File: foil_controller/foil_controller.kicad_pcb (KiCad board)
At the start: 2 copper layers, 90 x 110 mm, 18 parts, among them J1 programming_header, J2 pwr_in, J3 ultra sensor 1, J4 ultra sensor 1, SW1 SW_Push, SW2 SW_Push, SW3 SW_Push, SW4 SW_Push, U1 RS485_module, U2 L7805

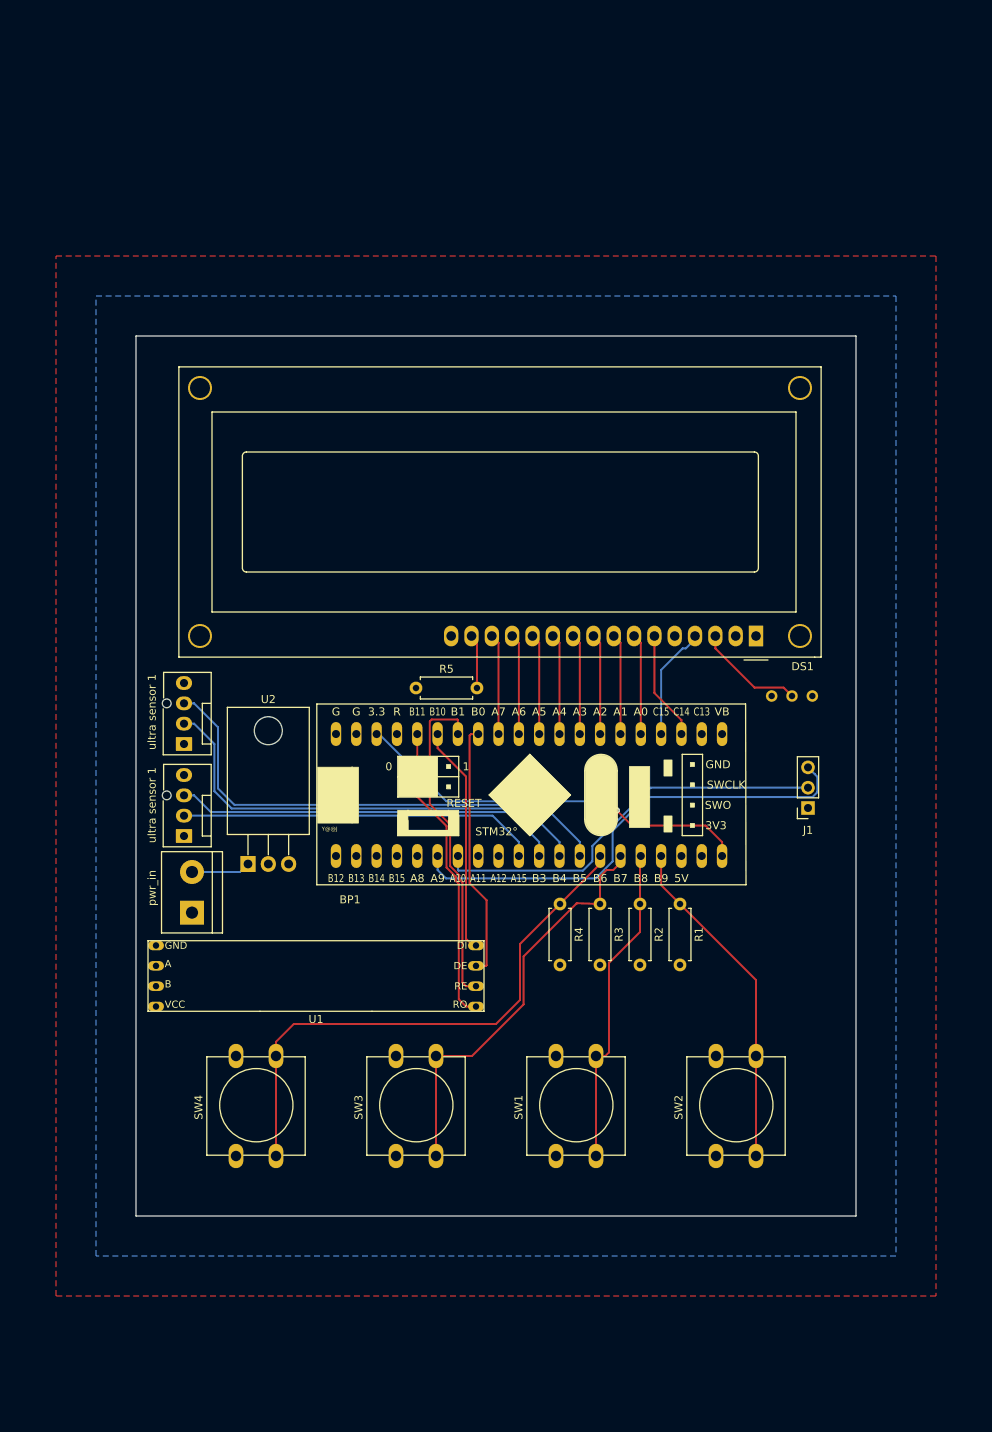
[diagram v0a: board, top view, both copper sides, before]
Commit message: controller v2 voor testvaart 1 mei
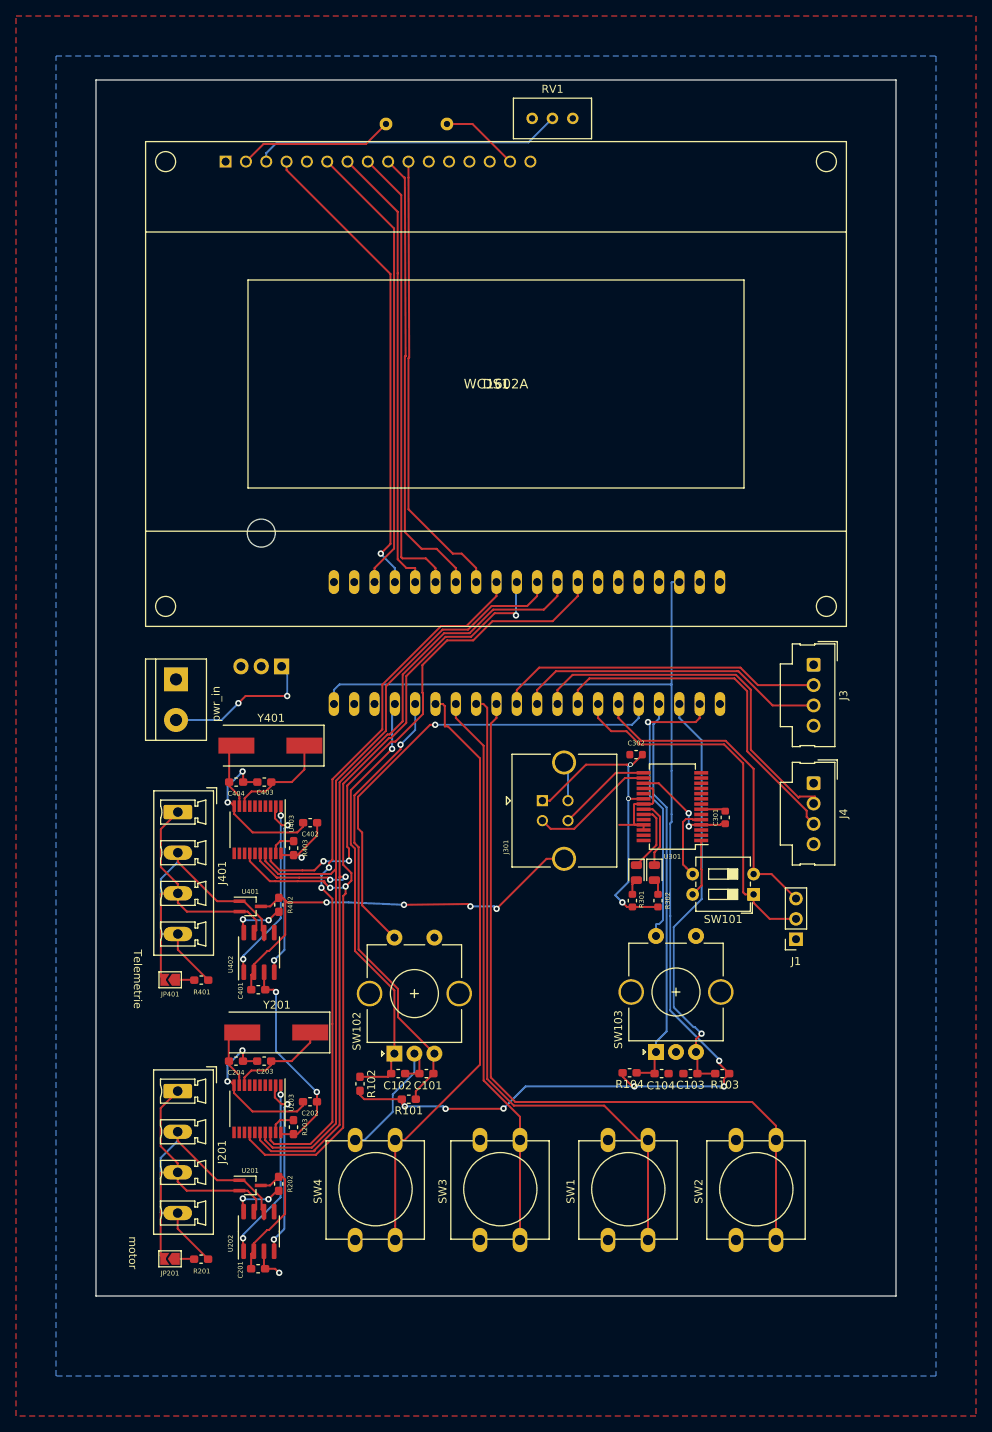
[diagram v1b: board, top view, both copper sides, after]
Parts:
- removed R1, R2, R3, R4: 10K, Resistor_THT:R_Axial_DIN0207_L6.3mm_D2.5mm_P7.62mm_Horizontal
- removed U1: RS485_module, stroom_shield:RS485_module
- added C101: 47nf, Capacitor_SMD:C_0603_1608Metric_Pad1.05x0.95mm_HandSolder, F.Cu at (36.3, 92.2)
- added C102: 47nf, Capacitor_SMD:C_0603_1608Metric_Pad1.05x0.95mm_HandSolder, F.Cu at (32.8, 92.2)
- added C103: 47nf, Capacitor_SMD:C_0603_1608Metric_Pad1.05x0.95mm_HandSolder, F.Cu at (69.3, 92.2)
- added C104: 47nf, Capacitor_SMD:C_0603_1608Metric_Pad1.05x0.95mm_HandSolder, F.Cu at (65.7, 92.2)
- added C201: 100nf, Capacitor_SMD:C_0603_1608Metric_Pad1.05x0.95mm_HandSolder, F.Cu at (15.3, 116.6)
- added C202: 100nf, Capacitor_SMD:C_0603_1608Metric_Pad1.05x0.95mm_HandSolder, F.Cu at (21.8, 95.7)
- added C203: 2pf, Capacitor_SMD:C_0603_1608Metric_Pad1.05x0.95mm_HandSolder, F.Cu at (16.0, 90.6)
- added C204: 2pf, Capacitor_SMD:C_0603_1608Metric_Pad1.05x0.95mm_HandSolder, F.Cu at (12.5, 90.6)
- added C301: 100nf, Capacitor_SMD:C_0603_1608Metric, F.Cu at (73.7, 60.2)
- added C302: 1uf, Capacitor_SMD:C_0603_1608Metric, F.Cu at (62.5, 52.3)
- added C401: 100nf, Capacitor_SMD:C_0603_1608Metric_Pad1.05x0.95mm_HandSolder, F.Cu at (15.3, 81.7)
- added C402: 100nf, Capacitor_SMD:C_0603_1608Metric_Pad1.05x0.95mm_HandSolder, F.Cu at (21.8, 60.8)
- added C403: 2pf, Capacitor_SMD:C_0603_1608Metric_Pad1.05x0.95mm_HandSolder, F.Cu at (16.0, 55.8)
- added C404: 2pf, Capacitor_SMD:C_0603_1608Metric_Pad1.05x0.95mm_HandSolder, F.Cu at (12.5, 55.8)
- added D301: TXLED, LED_SMD:LED_0805_2012Metric, F.Cu at (62.5, 67.1)
- added D302: RXLED, LED_SMD:LED_0805_2012Metric, F.Cu at (64.8, 67.1)
- added J201: can, Connector_Phoenix_MC_HighVoltage:PhoenixContact_MCV_1,5_4-G-5.08_1x04_P5.08mm_Vertical, F.Cu at (5.21, 94.4)
- added J301: USB_B, Connector_USB:USB_B_TE_5787834_Vertical, F.Cu at (50.8, 58.1)
- added J401: can, Connector_Phoenix_MC_HighVoltage:PhoenixContact_MCV_1,5_4-G-5.08_1x04_P5.08mm_Vertical, F.Cu at (5.23, 59.5)
- added JP201: termination, Jumper:SolderJumper-2_P1.3mm_Open_TrianglePad1.0x1.5mm, F.Cu at (4.25, 115.4)
- added JP401: termination, Jumper:SolderJumper-2_P1.3mm_Open_TrianglePad1.0x1.5mm, F.Cu at (4.27, 80.5)
- added R101: 10K, Resistor_SMD:R_0603_1608Metric_Pad1.05x0.95mm_HandSolder, F.Cu at (34.1, 95.4)
- added R102: 10K, Resistor_SMD:R_0603_1608Metric_Pad1.05x0.95mm_HandSolder, F.Cu at (28.0, 93.5)
- added R103: 10K, Resistor_SMD:R_0603_1608Metric_Pad1.05x0.95mm_HandSolder, F.Cu at (73.3, 92.2)
- added R104: 10K, Resistor_SMD:R_0603_1608Metric_Pad1.05x0.95mm_HandSolder, F.Cu at (61.7, 92.1)
- added R201: 120R, Resistor_SMD:R_0603_1608Metric_Pad1.05x0.95mm_HandSolder, F.Cu at (8.14, 115.4)
- added R202: 47K, Resistor_SMD:R_0603_1608Metric_Pad1.05x0.95mm_HandSolder, F.Cu at (17.8, 106.0)
- added R203: 10K, Resistor_SMD:R_0603_1608Metric_Pad1.05x0.95mm_HandSolder, F.Cu at (19.7, 98.9)
- added R301: 330R, Resistor_SMD:R_0603_1608Metric, F.Cu at (62.0, 70.6)
- added R302: 330R, Resistor_SMD:R_0603_1608Metric, F.Cu at (65.2, 70.6)
- added R401: 120R, Resistor_SMD:R_0603_1608Metric_Pad1.05x0.95mm_HandSolder, F.Cu at (8.16, 80.5)
- added R402: 47K, Resistor_SMD:R_0603_1608Metric_Pad1.05x0.95mm_HandSolder, F.Cu at (17.9, 71.1)
- added R403: 10K, Resistor_SMD:R_0603_1608Metric_Pad1.05x0.95mm_HandSolder, F.Cu at (19.7, 64.0)
- added SW101: SW_DIP_x02, Button_Switch_THT:SW_DIP_SPSTx02_Slide_6.7x6.64mm_W7.62mm_P2.54mm_LowProfile, F.Cu at (77.2, 69.8)
- added SW102: Encoder_1, Rotary_Encoder:RotaryEncoder_Alps_EC11E-Switch_Vertical_H20mm_CircularMountingHoles, F.Cu at (32.3, 89.7)
- added SW103: Encoder_2, Rotary_Encoder:RotaryEncoder_Alps_EC11E-Switch_Vertical_H20mm_CircularMountingHoles, F.Cu at (65.0, 89.5)
- added U201: PESD5V0L2UU_esd_diode, Package_TO_SOT_SMD:SOT-323_SC-70_Handsoldering, F.Cu at (14.3, 106.2)
- added U202: MCP2551-I-SN, Package_SO:SOIC-8_3.9x4.9mm_P1.27mm, F.Cu at (15.4, 111.9)
- added U203: MCP2515-xST, Package_SO:TSSOP-20_4.4x6.5mm_P0.65mm, F.Cu at (15.2, 96.6)
- added U301: FT232RL, Package_SO:SSOP-28_5.3x10.2mm_P0.65mm, F.Cu at (67.0, 58.8)
- added U401: PESD5V0L2UU_esd_diode, Package_TO_SOT_SMD:SOT-323_SC-70_Handsoldering, F.Cu at (14.3, 71.3)
- added U402: MCP2551-I-SN, Package_SO:SOIC-8_3.9x4.9mm_P1.27mm, F.Cu at (15.4, 77.0)
- added U403: MCP2515-xST, Package_SO:TSSOP-20_4.4x6.5mm_P0.65mm, F.Cu at (15.2, 61.7)
- added Y201: Crystal, Crystal:Crystal_SMD_HC49-SD, F.Cu at (17.5, 87.1)
- added Y401: Crystal, Crystal:Crystal_SMD_HC49-SD, F.Cu at (16.8, 51.2)
- BP1, R5, U2: moved to B.Cu
- DS1: footprint Display:WC1602A -> zonneboot_parts:WINSTAR-WH1604A
- J3, J4: footprint Connector:FanPinHeader_1x04_P2.54mm_Vertical -> Connector_Molex:Molex_SL_171971-0004_1x04_P2.54mm_Vertical
- RV1: moved to F.Cu
- moved J3 79.3 mm to (84.7, 41.1), turned to 270 degrees
- moved J4 79.0 mm to (84.7, 55.9), turned to 270 degrees
- moved RV1 78.2 mm to (54.6, -27.2)
- moved R5 70.6 mm to (31.2, -26.5)
- moved BP1 51.6 mm to (73.0, 46.0), turned to 180 degrees
- moved DS1 45.3 mm to (45.0, 6.00), turned to 0 degrees
- moved J2 29.2 mm to (5.00, 42.9), turned to 270 degrees
- moved U2 25.1 mm to (18.2, 41.3), turned to 180 degrees
- moved SW4 18.2 mm to (27.4, 113.0)
- moved J1 16.5 mm to (82.5, 75.4)
- moved SW3 14.8 mm to (43.0, 113.0)
- moved SW1 12.3 mm to (59.0, 113.0)
- moved SW2 10.8 mm to (75.0, 113.0)
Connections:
- BP1 pad 10: trig_2 -> echo_1
- BP1 pad 11: echo_2 -> trig_1
- BP1 pad 12: trig_1 -> btn_1
- BP1 pad 13: echo_1 -> btn_2
- BP1 pad 14: btn_4 -> btn_3
- BP1 pad 15: btn_3 -> btn_4
- BP1 pad 16: btn_2 -> /Encoder1_B
- BP1 pad 17: btn_1 -> /Encoder1_A
- BP1 pad 2: Net-(BP1-Pad2) -> /Encoder2_btn
- BP1 pad 29: Net-(BP1-Pad29) -> /Sheet60804332/can_spi_cs
- BP1 pad 3: Net-(BP1-Pad3) -> /Encoder2_B
- BP1 pad 30: Net-(BP1-Pad30) -> /Sheet60804332/can_spi_clk
- BP1 pad 31: Net-(BP1-Pad31) -> /Sheet60804332/can_spi_miso
- BP1 pad 32: Net-(BP1-Pad32) -> /Sheet60804332/can_spi_mosi
- BP1 pad 33: Net-(BP1-Pad33) -> /sheet60828324/can_spi_cs
- BP1 pad 4: Net-(BP1-Pad4) -> /Encoder2_A
- BP1 pad 5: Net-(BP1-Pad5) -> /Encoder1_btn
- BP1 pad 8: Net-(BP1-Pad8) -> echo_2
- BP1 pad 9: Net-(BP1-Pad9) -> trig_2
- DS1 pad 11: Net-(BP1-Pad29) -> Net-(DS1-Pad11)
- DS1 pad 12: Net-(BP1-Pad30) -> Net-(DS1-Pad12)
- DS1 pad 13: Net-(BP1-Pad31) -> Net-(DS1-Pad13)
- DS1 pad 14: Net-(BP1-Pad32) -> Net-(DS1-Pad14)
- SW1 pad 1: +5V -> GND
- SW2 pad 1: +5V -> GND
- SW3 pad 1: +5V -> GND
- SW4 pad 1: +5V -> GND
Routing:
- net GND: track 0.00 -> 151.8 mm, vias 0 -> 8
- net /Sheet60804332/can_spi_mosi: track 0.00 -> 111.3 mm, vias 0 -> 2
- net +3V3: track 51.0 -> 162.3 mm, vias 1 -> 6
- net /Sheet60804332/can_spi_clk: track 0.00 -> 111.3 mm, vias 0 -> 3
- net /Sheet60804332/can_spi_miso: track 0.00 -> 104.8 mm
- net /Sheet60804332/can_spi_cs: track 0.00 -> 89.0 mm, vias 0 -> 2
- net /sheet60828324/can_spi_cs: track 0.00 -> 65.3 mm, vias 0 -> 2
- net /Encoder1_btn: track 0.00 -> 60.4 mm, vias 0 -> 1
- net +5V: track 0.00 -> 58.9 mm, vias 0 -> 4
- net /Encoder1_B: track 0.00 -> 57.7 mm, vias 0 -> 1
- net btn_1: track 42.4 -> 99.4 mm
- net /Encoder1_A: track 0.00 -> 55.0 mm, vias 0 -> 1
- net /Encoder2_B: track 0.00 -> 52.9 mm, vias 0 -> 1
- net /Encoder2_A: track 0.00 -> 50.1 mm
- net Net-(BP1-Pad26): track 12.6 -> 57.8 mm
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- added copper zone on B.Cu, net +5V
- added copper zone on F.Cu, net GND
- removed copper zone on F.Cu, net +5V
- removed copper zone on B.Cu, net GND
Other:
- board size 90 x 110 mm -> 100 x 152 mm
- board text added: "Telemetrie"
- board text added: "motor"
